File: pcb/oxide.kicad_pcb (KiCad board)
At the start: 2 copper layers, 224.7 x 91.7 mm, 121 parts, among them SW1 SW_MX, SW10 SW_MX, SW11 SW_MX, SW12 SW_MX, SW13 SW_MX, SW14 SW_MX, SW15 SW_MX, SW16 SW_MX, SW17 SW_MX, SW18 SW_MX, SW19 SW_MX, SW2 SW_MX, SW20 SW_MX, SW21 SW_MX, SW22 SW_MX, SW23 SW_MX, SW24 SW_MX, SW25 SW_MX, SW26 SW_MX, SW27 SW_MX, SW28 SW_MX, SW29 SW_MX, SW3 SW_MX, SW30 SW_MX, SW31 SW_MX, SW32 SW_MX, SW33 SW_MX, SW34 SW_MX, SW35 SW_MX, SW36 SW_MX, SW37 SW_MX, SW38 SW_MX, SW39 SW_MX, SW4 SW_MX, SW40 SW_MX, SW41 SW_MX, SW42 SW_MX, SW43 SW_MX, SW44 SW_MX, SW45 SW_MX, SW46 SW_MX, SW47 SW_MX, SW48 SW_MX, SW49 SW_MX, SW5 SW_MX, SW50 SW_MX, SW51 SW_MX, SW52 SW_MX, SW53 SW_MX, SW54 SW_MX, SW55 SW_MX, SW56 SW_MX, SW57 SW_MX, SW58 SW_MX, SW59 SW_MX, SW6 SW_MX, SW60 SW_MX, SW7 SW_MX, SW8 SW_MX, SW9 SW_MX

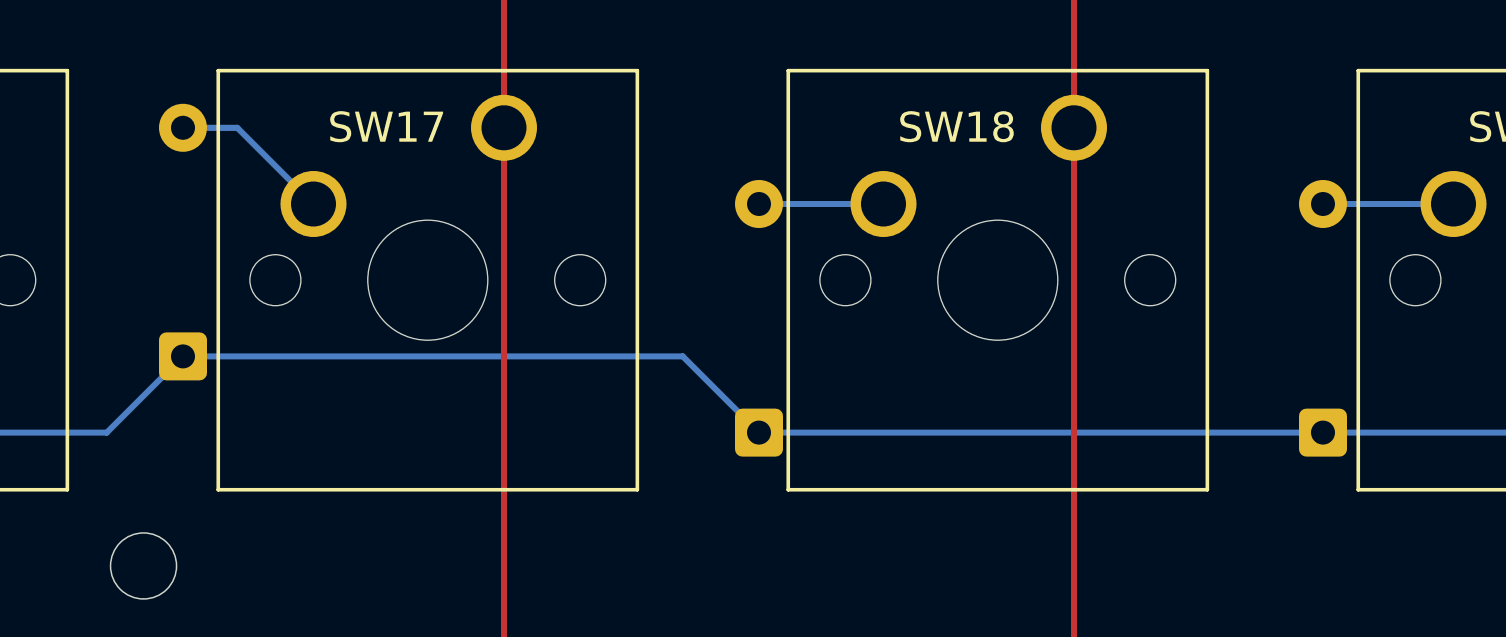
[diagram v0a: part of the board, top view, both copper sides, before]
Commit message: Fix diode position
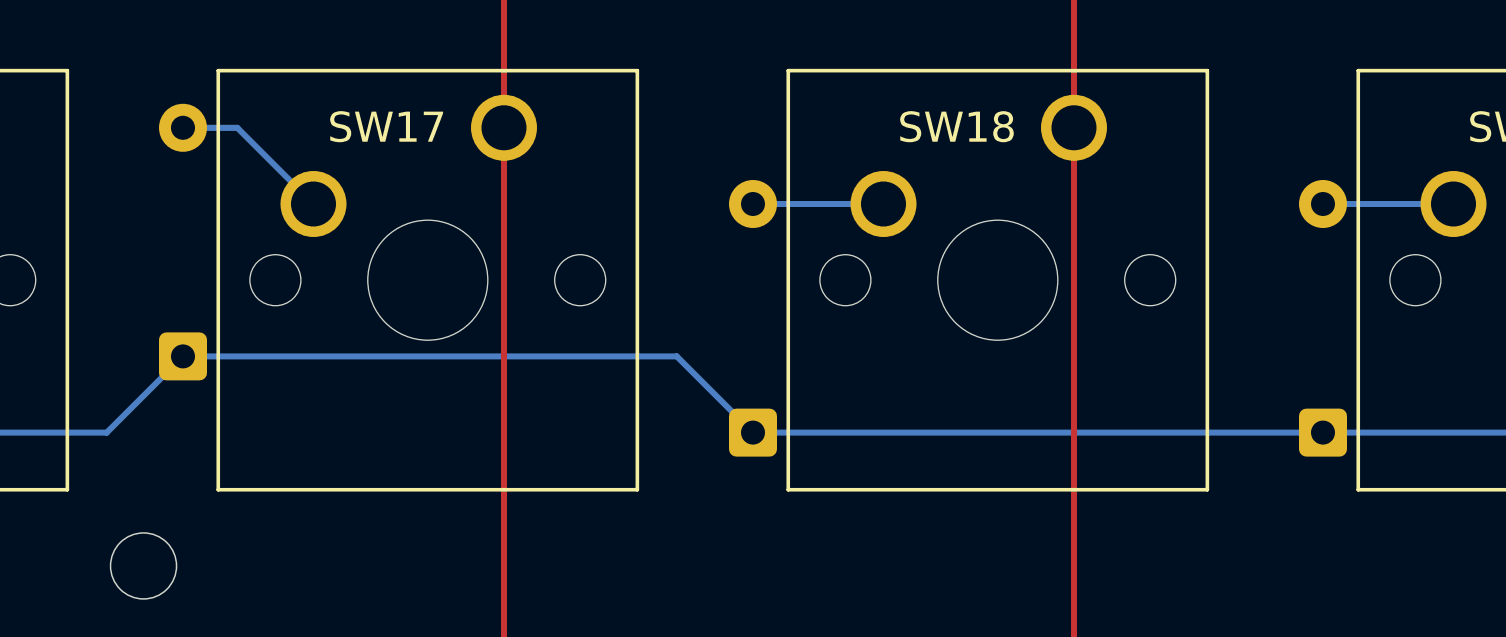
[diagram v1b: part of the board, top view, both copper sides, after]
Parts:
- moved D18 0.20 mm to (132.3, 118.7)
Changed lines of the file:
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@@
 		(capping no)
 		(filling no)
-		(zone_defaults)
 		(pcbplotparams
 			(layerselection 0x00000000_00000000_55555555_5755f5ff)
@@
 	(footprint "Diode_THT:D_DO-35_SOD27_P7.62mm_Horizontal"
 		(layer "B.Cu")
-		(at 132.5 118.66 90)
+		(at 132.3 118.66 90)
 		(descr "Diode, DO-35_SOD27 series, Axial, Horizontal, pin pitch=7.62mm, length*diameter=4*2mm^2, http://www.diodes.com/_files/packages/DO-35.pdf")
 		(tags "Diode DO-35_SOD27 series Axial Horizontal pin pitch 7.62mm  length 4mm diameter 2mm")
@@
 	)
 	(segment
-		(start 132.5 111.04)
+		(start 132.3 111.04)
 		(end 136.65 111.04)
 		(width 0.2)
@@
 	)
 	(segment
+		(start 129.76 116.12)
+		(end 132.3 118.66)
+		(width 0.2)
+		(layer "B.Cu")
+		(net "ROW1")
+	)
+	(segment
 		(start 110.76 118.66)
 		(end 113.3 116.12)
@@
 	)
 	(segment
-		(start 113.3 116.12)
-		(end 129.96 116.12)
-		(width 0.2)
-		(layer "B.Cu")
-		(net "ROW1")
-	)
-	(segment
 		(start 186.76 118.66)
 		(end 189.3 116.12)
@@
 	)
 	(segment
-		(start 246.3 116.12)
-		(end 229.84 116.12)
+		(start 113.3 116.12)
+		(end 129.76 116.12)
 		(width 0.2)
 		(layer "B.Cu")
@@
 	)
 	(segment
-		(start 129.96 116.12)
-		(end 132.5 118.66)
+		(start 132.3 118.66)
+		(end 151.3 118.66)
 		(width 0.2)
 		(layer "B.Cu")
@@
 	)
 	(segment
-		(start 170.3 118.66)
-		(end 151.3 118.66)
+		(start 246.3 116.12)
+		(end 229.84 116.12)
 		(width 0.2)
 		(layer "B.Cu")
@@
 	)
 	(segment
-		(start 132.5 118.66)
+		(start 170.3 118.66)
 		(end 151.3 118.66)
 		(width 0.2)
